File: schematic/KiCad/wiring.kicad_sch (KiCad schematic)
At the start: 31 parts, among them SW1 Manual/Auto, SW2 Pulse, U1 74LS08, U10 74LS173, U11 74LS173, U12 74LS86, U13 74LS86, U14 74LS283, U15 74LS283, U16 74LS245, U2 74LS32, U3 NE555P, U4 NE555P, U5 NE555P, U6 74LS173, U7 74LS04, U8 74LS173, U9 74LS245

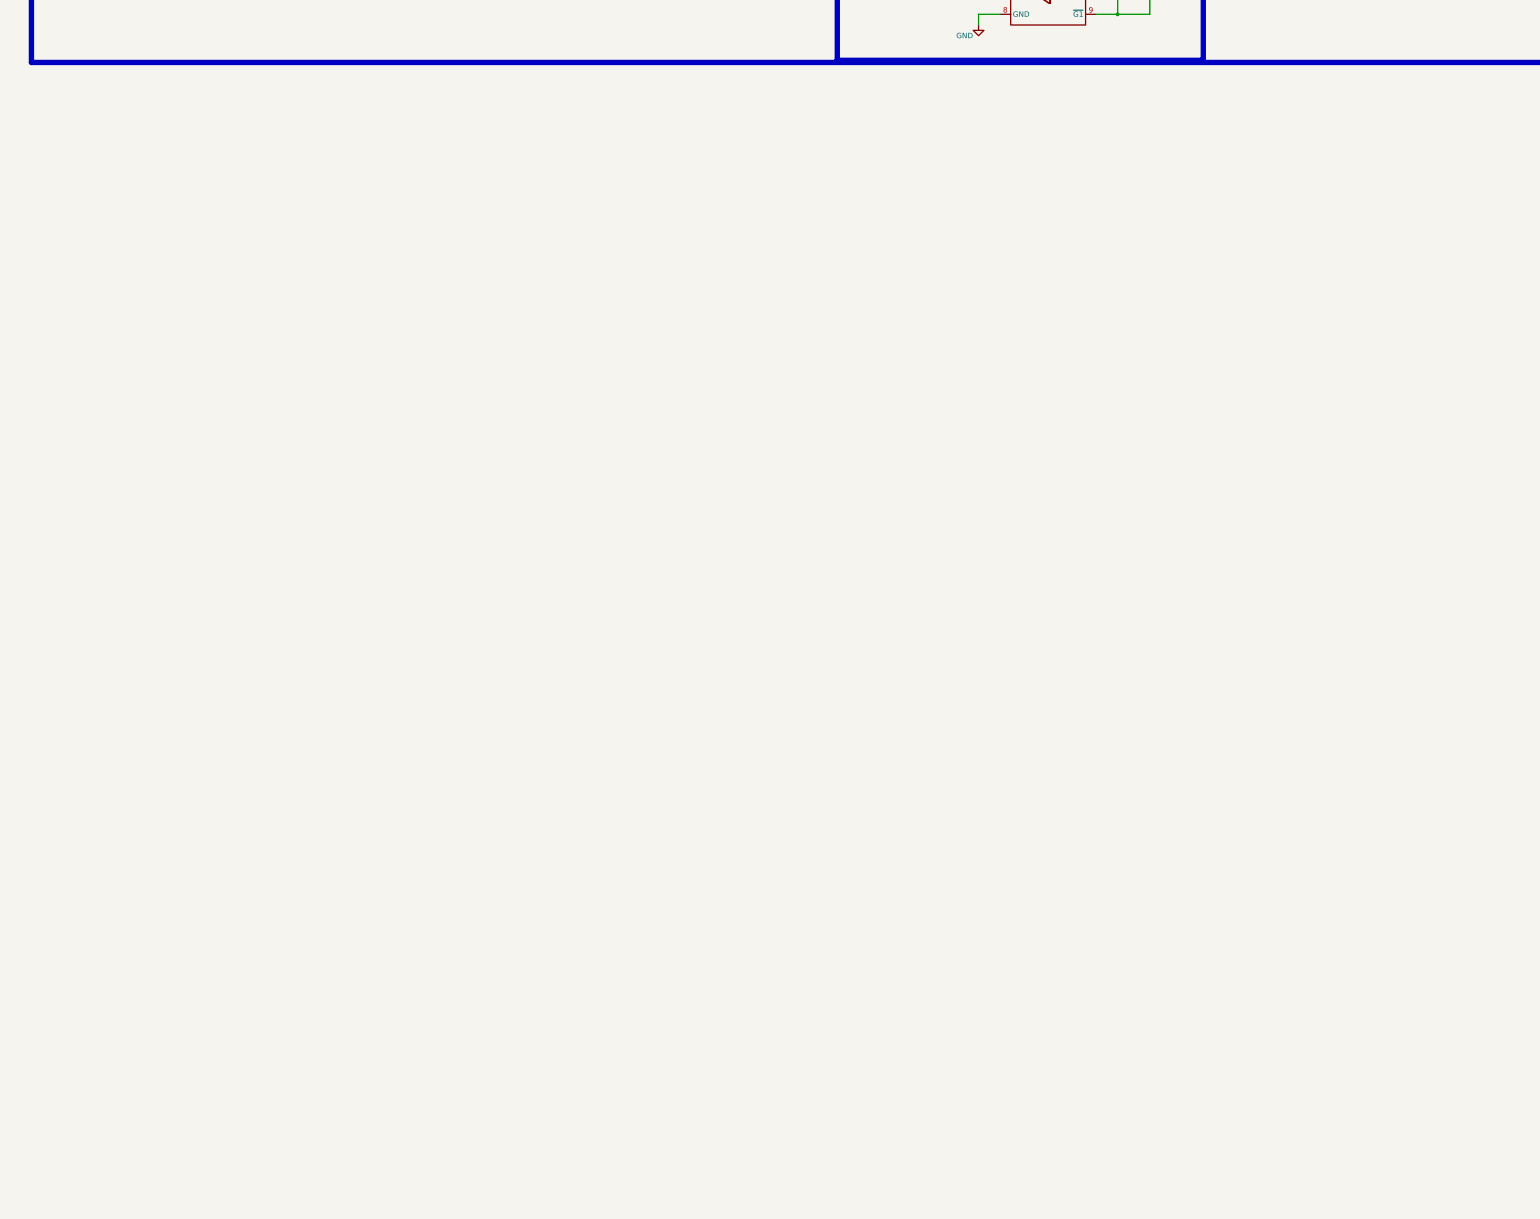
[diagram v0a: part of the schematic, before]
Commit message: Add files via upload
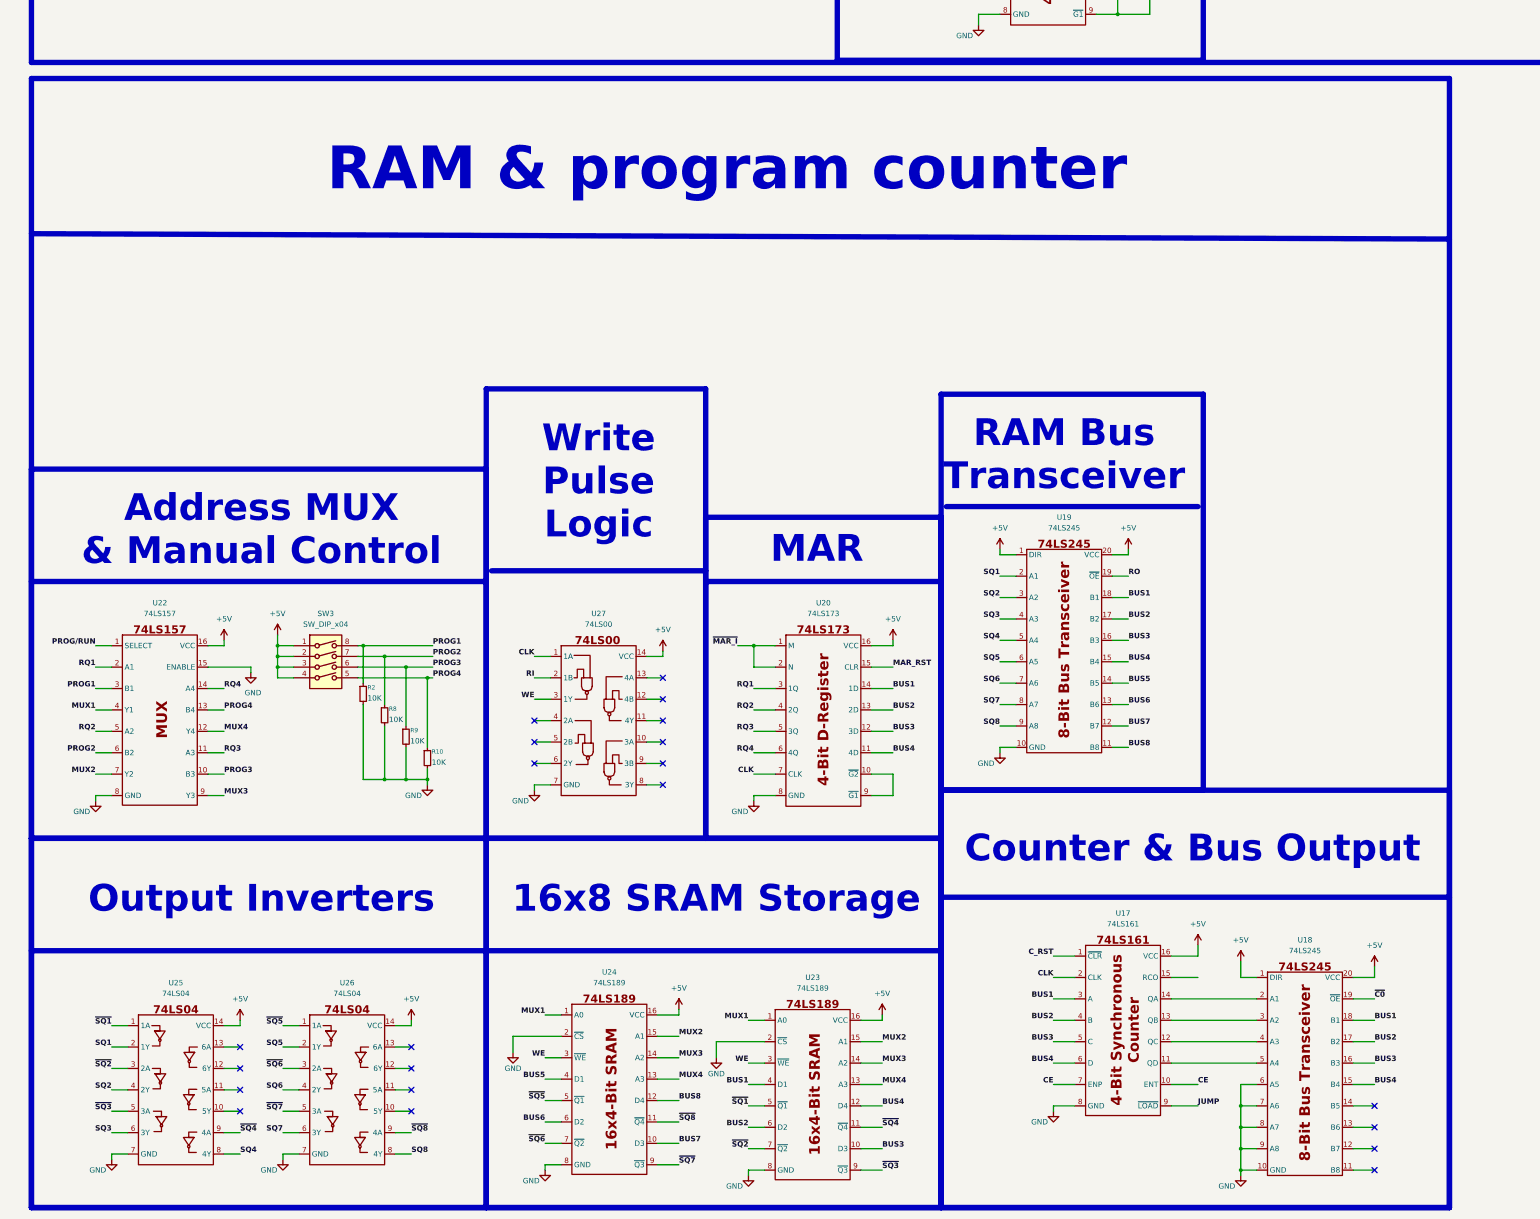
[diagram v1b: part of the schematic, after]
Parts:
- added R10, R2, R8, R9: 10K, symbol Device:R_Small
- added SW3: SW_DIP_x04, symbol Switch:SW_DIP_x04
- added U17: 74LS161, symbol 8-bit ICs:74LS161
- added U18, U19: 74LS245, symbol 8-bit ICs:74LS245
- added U20: 74LS173, symbol 8-bit ICs:74LS173
- added U22: 74LS157, symbol 8-bit ICs:74LS157
- added U23, U24: 74LS189, symbol 8-bit ICs:74LS189
- added U25, U26: 74LS04, symbol 8-bit ICs:74LS04
- added U27: 74LS00, symbol 8-bit ICs:74LS00
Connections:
- net +5V: now also SW3.1, SW3.2, SW3.3, SW3.4, U17.16 (VCC), U18.1 (DIR), U18.20 (VCC), U19.1 (DIR), U19.20 (VCC), U20.16 (VCC), U22.16 (VCC), U23.16 (VCC), U24.16 (VCC), U25.14 (VCC), U26.14 (VCC), U27.14 (VCC)
- net BUS1: now also U17.3 (A), U18.18 (B1), U19.18 (B1), U20.14 (1D), U23.4 (D1)
- net BUS2: now also U17.4 (B), U18.17 (B2), U19.17 (B2), U20.13 (2D), U23.6 (D2)
- net BUS3: now also U17.5 (C), U18.16 (B3), U19.16 (B3), U20.12 (3D), U23.10 (D3)
- net BUS4: now also U17.6 (D), U18.15 (B4), U19.15 (B4), U20.11 (4D), U23.12 (D4)
- net BUS5: now also U19.14 (B5), U24.4 (D1)
- net BUS6: now also U19.13 (B6), U24.6 (D2)
- net BUS7: now also U19.12 (B7), U24.10 (D3)
- net BUS8: now also U19.11 (B8), U24.12 (D4)
- net CLK: now also U17.2 (CLK), U20.7 (CLK), U27.1 (1A)
- net GND: now also R10.2, R2.2, R8.2, R9.2, U17.8 (GND), U18.10 (GND), U18.6 (A5), U18.7 (A6), U18.8 (A7), U18.9 (A8), U19.10 (GND), U20.8 (GND), U22.15 (ENABLE), U22.8 (GND), U23.2 (~{CS}), U23.8 (GND), U24.2 (~{CS}), U24.8 (GND), U25.7 (GND), U26.7 (GND), U27.7 (GND)
- new net: U17.14 (QA), U18.2 (A1)
- new net: U17.13 (QB), U18.3 (A2)
- new net: U17.12 (QC), U18.4 (A3)
- new net: U17.11 (QD), U18.5 (A4)
- new net: U20.10 (~{G2}), U20.9 (~{G1})
- new net CE: U17.10 (ENT), U17.7 (ENP)
- new net C_RST: U17.1 (~{CLR})
- new net JUMP: U17.9 (~{LOAD})
- new net MAR_RST: U20.15 (CLR)
- new net MUX1: U22.4 (Y1), U23.1 (A0), U24.1 (A0)
- new net MUX2: U22.7 (Y2), U23.15 (A1), U24.15 (A1)
- new net MUX3: U22.9 (Y3), U23.14 (A2), U24.14 (A2)
- new net MUX4: U22.12 (Y4), U23.13 (A3), U24.13 (A3)
- new net PROG1: R2.1, SW3.8, U22.3 (B1)
- new net PROG2: R8.1, SW3.7, U22.6 (B2)
- new net PROG3: R9.1, SW3.6, U22.10 (B3)
- new net PROG4: R10.1, SW3.5, U22.13 (B4)
- new net PROG/RUN: U22.1 (SELECT)
- new net RI: U27.2 (1B)
- new net RO: U19.19 (~{OE})
- new net RQ1: U20.3 (1Q), U22.2 (A1)
- new net RQ2: U20.4 (2Q), U22.5 (A2)
- new net RQ3: U20.5 (3Q), U22.11 (A3)
- new net RQ4: U20.6 (4Q), U22.14 (A4)
- new net SQ1: U19.2 (A1), U25.2 (1Y)
- new net SQ2: U19.3 (A2), U25.4 (2Y)
- new net SQ3: U19.4 (A3), U25.6 (3Y)
- new net SQ4: U19.5 (A4), U25.8 (4Y)
- new net SQ5: U19.6 (A5), U26.2 (1Y)
- new net SQ6: U19.7 (A6), U26.4 (2Y)
- new net SQ7: U19.8 (A7), U26.6 (3Y)
- new net SQ8: U19.9 (A8), U26.8 (4Y)
- new net WE: U23.3 (~{WE}), U24.3 (~{WE}), U27.3 (1Y)
- new net ~{C0}: U18.19 (~{OE})
- new net ~{MAR_I}: U20.1 (M), U20.2 (N)
- new net ~{SQ1}: U23.5 (~{Q1}), U25.1 (1A)
- new net ~{SQ2}: U23.7 (~{Q2}), U25.3 (2A)
- new net ~{SQ3}: U23.9 (~{Q3}), U25.5 (3A)
- new net ~{SQ4}: U23.11 (~{Q4}), U25.9 (4A)
- new net ~{SQ5}: U24.5 (~{Q1}), U26.1 (1A)
- new net ~{SQ6}: U24.7 (~{Q2}), U26.3 (2A)
- new net ~{SQ7}: U24.9 (~{Q3}), U26.5 (3A)
- new net ~{SQ8}: U24.11 (~{Q4}), U26.9 (4A)
- no-connect marks 21 -> 42
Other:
- note added: "16x8 SRAM Storage"
- note added: "Address MUX & Manual Control"
- note added: "Counter & Bus Output"
- note added: "MAR"
- note added: "Output Inverters"
- note added: "RAM & program counter"
- note added: "RAM Bus Transceiver"
- note added: "Write Pulse Logic"
